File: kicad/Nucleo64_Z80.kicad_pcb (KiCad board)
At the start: 2 copper layers, 68.6 x 57.2 mm, 28 parts, among them J1 Conn_01x20_Pin, J2 Conn_01x20_Pin, J3 Qwiic_connector, J4 SD Card slot, J5 SD Card slot, U2 AS6C4008-55PCN, U3 Z80CPU, U4 74LS125

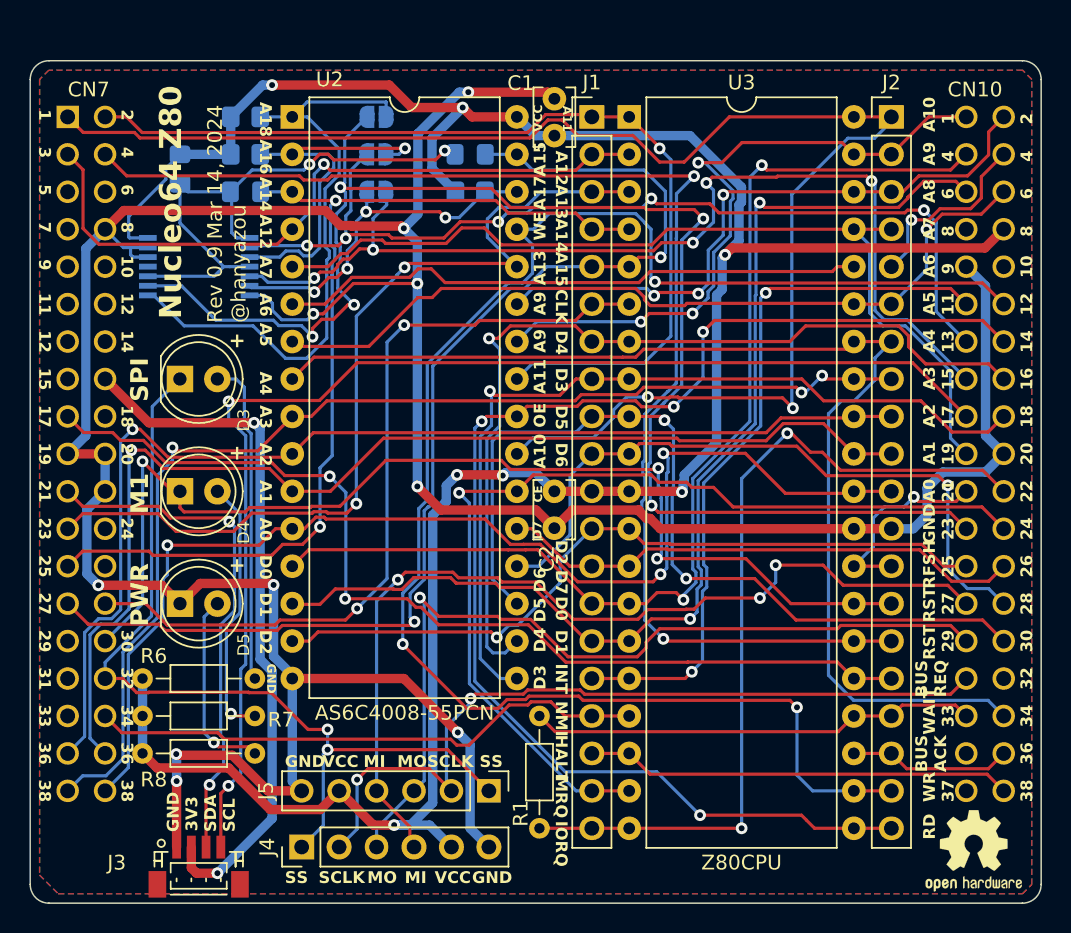
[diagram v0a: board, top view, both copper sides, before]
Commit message: Add Nucleo64_Z80 PCB revision 1.0
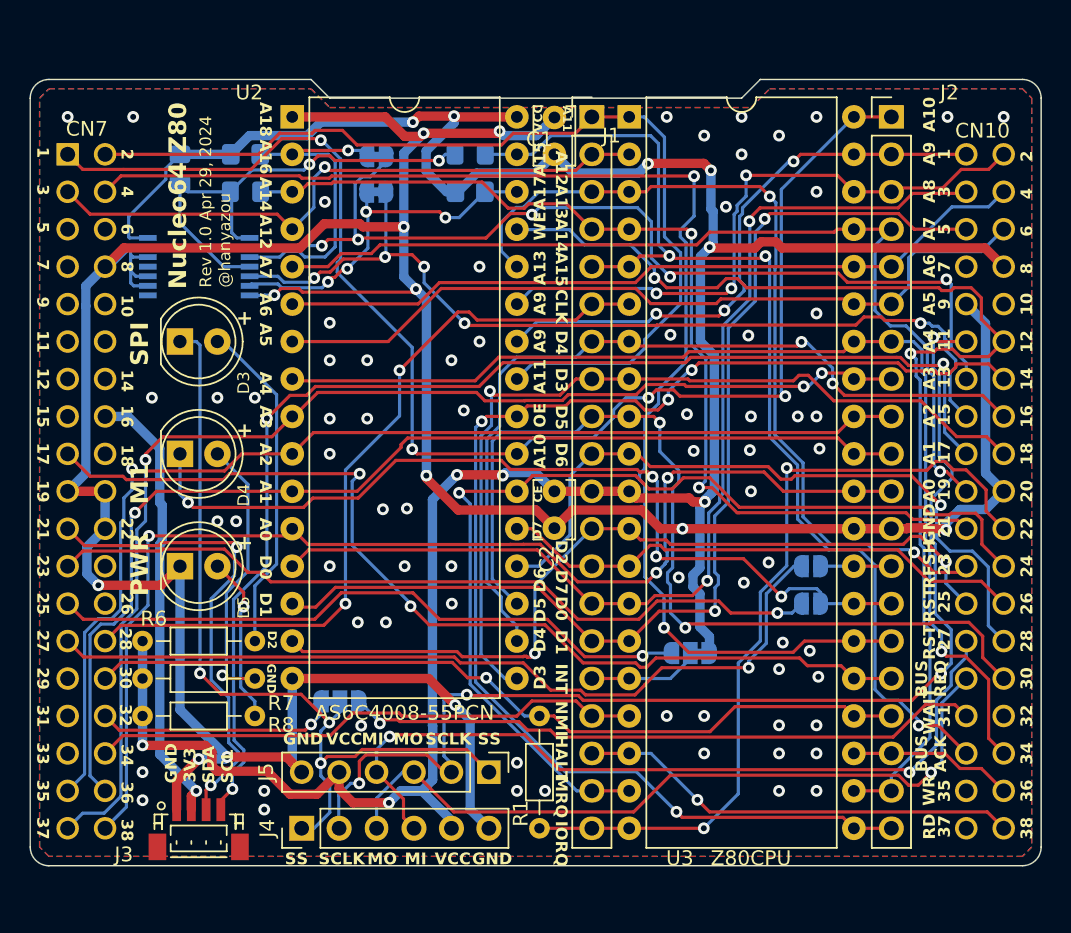
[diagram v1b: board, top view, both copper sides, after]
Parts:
- removed R5: 10K, Resistor_SMD:R_0805_2012Metric_Pad1.20x1.40mm_HandSolder
- added JP4: SolderJumper_2_Open, Jumper:SolderJumper-2_P1.3mm_Open_RoundedPad1.0x1.5mm, B.Cu at (158.4, 127.0)
- added JP5: SolderJumper_2_Bridged, Jumper:SolderJumper-2_P1.3mm_Bridged_RoundedPad1.0x1.5mm, B.Cu at (128.9, 99.2)
- added JP6: SolderJumper_2_Bridged, Jumper:SolderJumper-2_P1.3mm_Bridged_RoundedPad1.0x1.5mm, B.Cu at (128.9, 101.6)
- C1, C2: value C_Small -> 0.1uF
- JP1, JP2: value SolderJumper_2_Open -> SolderJumper_3_Bridged12; footprint Jumper:SolderJumper-2_P1.3mm_Open_RoundedPad1.0x1.5mm -> Jumper:SolderJumper-3_P1.3mm_Bridged12_RoundedPad1.0x1.5mm_NumberLabels
- R1: value R_Small -> 200
- REF**: moved to B.Cu
- moved REF** 55.0 mm to (128.4, 109.6), turned to -90 degrees
- moved JP3 44.3 mm to (158.4, 129.5)
- moved JP2 37.9 mm to (150.2, 132.9)
- moved JP1 37.2 mm to (126.4, 136.2)
- moved D4 2.54 mm to (115.6, 119.4)
- moved D3 2.54 mm to (115.6, 111.8)
- moved D5 2.54 mm to (115.6, 127.0)
- moved J3 2.54 mm to (116.8, 144.8)
- moved R6 2.54 mm to (113.0, 132.1)
- moved R7 2.54 mm to (113.0, 134.6)
- moved R8 2.54 mm to (113.0, 137.2)
- moved U1 2.54 mm to (139.7, 108.6)
- moved J4 1.27 mm to (123.8, 144.8)
- moved J5 1.27 mm to (136.5, 141.0)
- moved C1 1.27 mm to (141.0, 99.1)
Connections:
- JP1 pad 1: BANK_SEL0 -> PA4
- JP1 pad 2: A16 -> ~{SPI1_SS}
- JP2 pad 1: BANK_SEL1 -> VCC
- JP2 pad 2: A17 -> ~{INT}
- JP3 pad 1: BANK_SEL2 -> PC13
- JP3 pad 2: A18 -> ~{M1}
- U1 pad CN10_11: ~{INT} -> SPI1_SCLK
- U1 pad CN10_21: ~{RFSH} -> A14
- U1 pad CN10_23: BANK_SEL2 -> A13
- U1 pad CN10_31: SPI1_SCLK -> PB3
- U1 pad CN10_33: ~{WAIT} -> A15
- U1 pad CN7_23: A13 -> PC13
- U1 pad CN7_25: A14 -> PC14
- U1 pad CN7_27: A15 -> PC15
- U1 pad CN7_30: ~{M1} -> ~{WAIT}
- U1 pad CN7_32: ~{SPI1_SS} -> PA4
- U2 pad 1: A18 -> GND
- U4 pad 10: Net-(D1-A) -> GND
- U4 pad 8: A18 -> unconnected-(U4-Pad8)
- U4 pad 9: BANK_SEL2 -> GND
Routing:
- net BANK_SEL2: track 99.8 -> 0.00 mm, vias 5 -> 0
- net PC15: track 0.00 -> 57.2 mm, vias 0 -> 1
- net PC13: track 0.00 -> 53.3 mm, vias 0 -> 1
- net PC14: track 0.00 -> 44.0 mm, vias 0 -> 1
- net PB3: track 0.00 -> 43.7 mm, vias 0 -> 1
- net A18: track 42.0 -> 0.00 mm
- net ~{INT}: track 49.1 -> 7.62 mm, vias 2 -> 0
- net ~{WR}: track 111.4 -> 79.0 mm, vias 3 -> 2
- net ~{WAIT}: track 30.4 -> 56.7 mm, vias 0 -> 1
- net SPI1_SCLK: track 53.9 -> 79.4 mm, vias 2 -> 4
- net 3V3: track 47.3 -> 30.4 mm, vias 2 -> 1
- net PA4: track 0.00 -> 16.4 mm, vias 0 -> 1
- net VCC: track 173.8 -> 189.7 mm, vias 7 -> 10
- net ~{M1}: track 75.6 -> 60.7 mm, vias 3 -> 4
- net A10: track 104.1 -> 93.6 mm, vias 2 -> 4
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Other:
- board size 68.6 x 57.2 mm -> 68.6 x 53.3 mm
- board text added: "35"
- board text added: "Rev 1.0 Apr 29, 2024 @hanyazou"
- board text added: "https://github.com/hanyazou/Nucleo64_Z80"
- board text removed: "Rev 0.9 Mar 14, 2024 @hanyazou"
